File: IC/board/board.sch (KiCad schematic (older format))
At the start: 34 parts, among them Q1 IRLZ44N, SW1 SW_Push, SW2 SW_Push, SW3 SW_Push, SW4 SW_Push, SW5 SW_Push, U1 L7805, U2 ATmega328P-PU, Y1 16Mhz

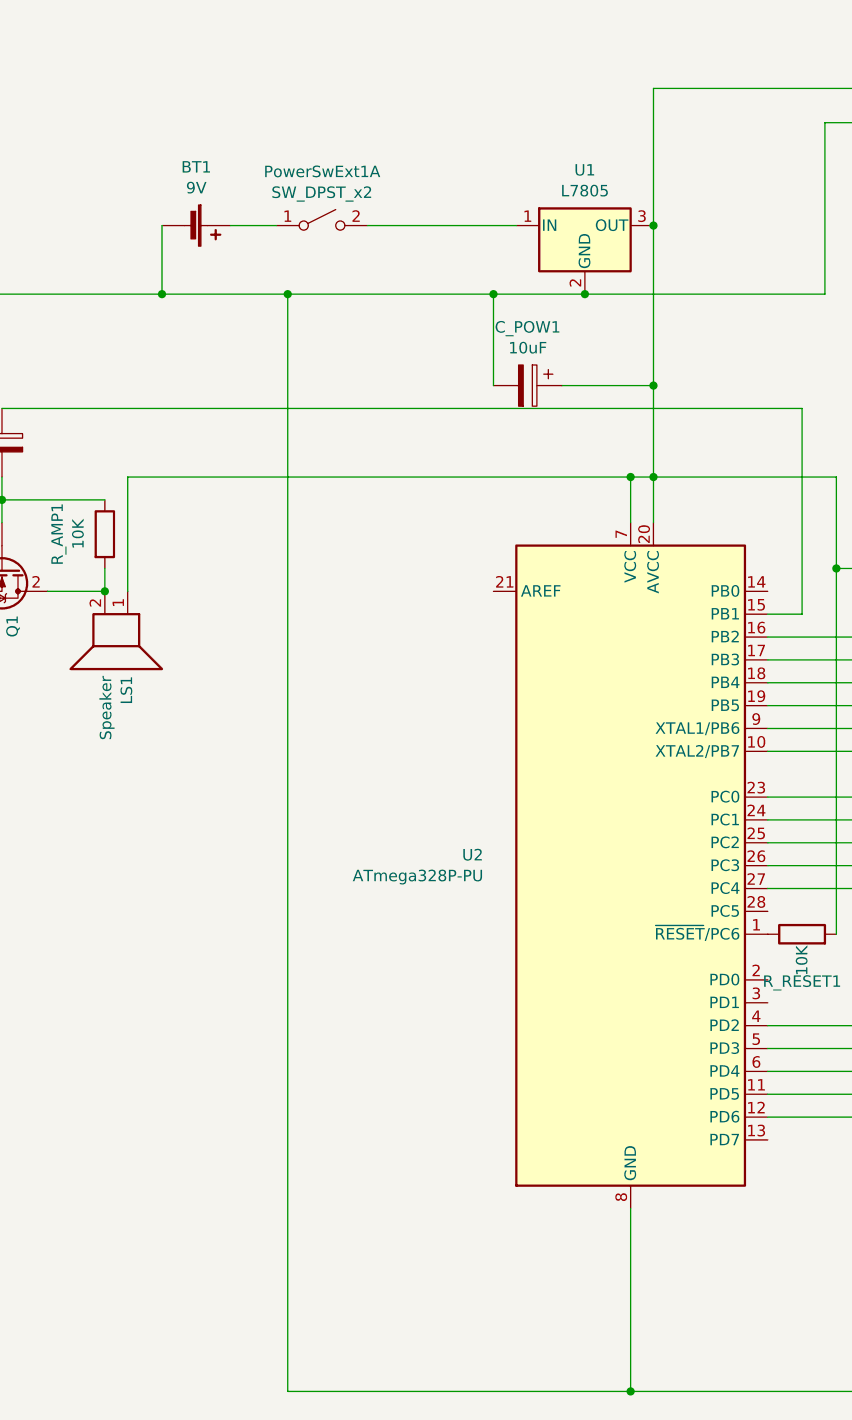
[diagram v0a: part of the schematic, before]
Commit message: Update
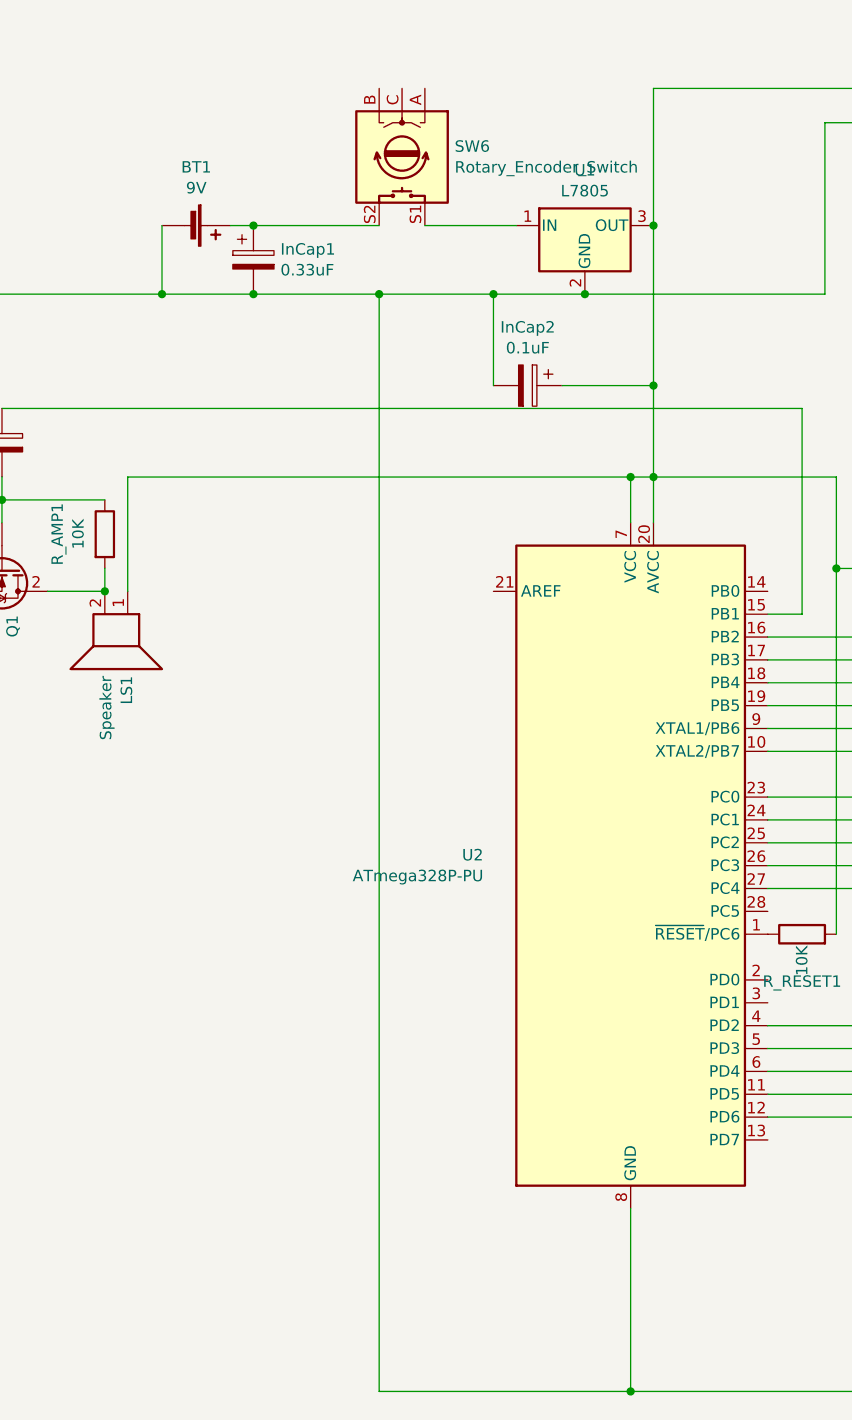
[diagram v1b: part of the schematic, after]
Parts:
- removed PowerSwExt1: SW_DPST_x2, Connector_JST:JST_EH_B2B-EH-A_1x02_P2.50mm_Vertical, symbol Switch:SW_DPST_x2
- added InCap1: 0.33uF, Capacitor_THT:CP_Radial_D5.0mm_P2.50mm, symbol Device:CP
- added SW6: Rotary_Encoder_Switch, Connector_JST:JST_EH_B5B-EH-A_1x05_P2.50mm_Vertical, symbol Device:Rotary_Encoder_Switch
- InCap2: renamed from C_POW1; value 10uF -> 0.1uF; footprint Capacitor_THT:CP_Radial_D6.3mm_P2.50mm -> Capacitor_THT:CP_Radial_D5.0mm_P2.50mm
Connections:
- net at BT1.1 (+): now also InCap1.1, SW6.S2
- net at BT1.2 (-), C1_CRY1.2, C2_CRY1.2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: now also InCap1.2
- net at U1.1 (IN): now also SW6.S1
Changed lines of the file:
@@
 	4550 1850 4950 1850
 $Comp
-L Device:CP C_POW1
+L Device:CP InCap2
 U 1 1 623A7132
 P 4400 1850
-F 0 "C_POW1" V 4145 1850 50  0000 C CNN
-F 1 "10uF" V 4236 1850 50  0000 C CNN
-F 2 "Capacitor_THT:CP_Radial_D6.3mm_P2.50mm" H 4438 1700 50  0001 C CNN
+F 0 "InCap2" V 4145 1850 50  0000 C CNN
+F 1 "0.1uF" V 4236 1850 50  0000 C CNN
+F 2 "Capacitor_THT:CP_Radial_D5.0mm_P2.50mm" H 4438 1700 50  0001 C CNN
 F 3 "~" H 4400 1850 50  0001 C CNN
 	1    4400 1850
@@
 $EndComp
 Wire Wire Line
-	4250 1450 3350 1450
+	4250 1450 3750 1450
 Connection ~ 4250 1450
 Wire Wire Line
@@
 	4950 1850 4950 1150
 Connection ~ 4950 1850
-Connection ~ 3350 1450
 Wire Wire Line
 	4650 1450 4250 1450
@@
 $EndComp
 Wire Wire Line
-	4850 6250 3350 6250
+	4850 6250 3750 6250
 Wire Wire Line
 	4850 5450 4850 6250
@@
 	2100 1950 5600 1950
 Wire Wire Line
-	3350 1450 3350 6250
+	3750 1450 3750 6250
 Wire Wire Line
 	1600 1450 1600 2750
@@
 	2800 1450 1600 1450
 Wire Wire Line
-	2800 1450 3350 1450
-Wire Wire Line
-	3300 1150 3100 1150
-$Comp
-L Switch:SW_DPST_x2 PowerSwExt1
-U 1 1 62AC8AE8
-P 3500 1150
-F 0 "PowerSwExt1" H 3500 1385 50  0000 C CNN
-F 1 "SW_DPST_x2" H 3500 1294 50  0000 C CNN
-F 2 "Connector_JST:JST_EH_B2B-EH-A_1x02_P2.50mm_Vertical" H 3500 1150 50  0001 C CNN
-F 3 "~" H 3500 1150 50  0001 C CNN
-	1    3500 1150
-	1    0    0    -1
-$EndComp
+	2800 1450 3200 1450
 Wire Wire Line
 	6400 2650 5750 2650
@@
 Wire Wire Line
 	7600 700  7600 2550
-Wire Wire Line
-	3700 1150 4350 1150
+$Comp
+L Device:CP InCap1
+U 1 1 6233B054
+P 3200 1300
+F 0 "InCap1" H 3318 1346 50  0000 L CNN
+F 1 "0.33uF" H 3318 1255 50  0000 L CNN
+F 2 "Capacitor_THT:CP_Radial_D5.0mm_P2.50mm" H 3238 1150 50  0001 C CNN
+F 3 "~" H 3200 1300 50  0001 C CNN
+	1    3200 1300
+	1    0    0    -1
+$EndComp
+Connection ~ 3200 1150
+Wire Wire Line
+	3200 1150 3100 1150
+Connection ~ 3200 1450
+Connection ~ 3750 1450
+Wire Wire Line
+	3200 1450 3750 1450
+$Comp
+L Device:Rotary_Encoder_Switch SW6
+U 1 1 62300B3A
+P 3850 850
+F 0 "SW6" V 3804 1080 50  0000 L CNN
+F 1 "Rotary_Encoder_Switch" V 3895 1080 50  0000 L CNN
+F 2 "Connector_JST:JST_EH_B5B-EH-A_1x05_P2.50mm_Vertical" H 3700 1010 50  0001 C CNN
+F 3 "~" H 3850 1110 50  0001 C CNN
+	1    3850 850
+	0    1    1    0
+$EndComp
+Wire Wire Line
+	3950 1150 4350 1150
+Wire Wire Line
+	3200 1150 3750 1150
 $EndSCHEMATC
